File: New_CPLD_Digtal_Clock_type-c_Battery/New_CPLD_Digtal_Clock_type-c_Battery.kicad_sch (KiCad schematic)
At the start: 43 parts, among them J1 Conn_02x05_Odd_Even, J2 Conn_01x15, J3 Conn_01x15, P1 USB_C_Plug_USB2.0, Q1 CS9013, Q2 CS9013, Q3 CS9013, Q4 CS9013, SW1 SW_Push, SW2 SW_Push, SW3 SW_Push, SW4 SW_Nidec_CAS-120A1, U1 4_Digits_7Seg_CC, U2 LD1117V33, Y1 CXO_DIP8

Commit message: Add files via upload
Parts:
- added C7, C9: 0.1uF, Capacitor_SMD:C_0201_0603Metric, symbol Device:C
- added C8: 10uF, Capacitor_SMD:C_0201_0603Metric, symbol Device:C
- added D2, D3: LED, LED_SMD:LED_PLCC_2835, symbol Device:LED
- added Q5: FS8205A, SOP65P640X120-8N, symbol FS8205A:FS8205A
- added R21, R22, R25: 1k, Resistor_SMD:R_0201_0603Metric, symbol Device:R_US
- added R23: 100, Resistor_SMD:R_0201_0603Metric, symbol Device:R_US
- added R26: 1.2k, Resistor_SMD:R_0201_0603Metric, symbol Device:R_US
- added U1: EPM3064ATC100-7N, EPM3064:PLCC127P1765X1765X457-44N, symbol EPM3064:EPM3064ATC100-7N
- added U4: TP4056-42-ESOP8, Package_SO:SOIC-8-1EP_3.9x4.9mm_P1.27mm_EP2.41x3.3mm_ThermalVias, symbol TP4056:TP4056-42-ESOP8
- added U5: DW01A, Package_TO_SOT_SMD:SOT-23-6, symbol Battery_Management:DW01A
- BT1: value Battery -> 3.7V
- C1: value C -> 10uF; footprint (none) -> Capacitor_SMD:C_0201_0603Metric; Voltage (none) -> 25V
- C2, C3, C4, C5, C6: footprint (none) -> Capacitor_SMD:C_0201_0603Metric
- D1: footprint (none) -> LED_SMD:LED_PLCC_2835
- J1: footprint (none) -> Connector_IDC:IDC-Header_2x03_P2.54mm_Vertical
- J2, J3: footprint (none) -> Connector_PinHeader_1.00mm:PinHeader_1x15_P1.00mm_Vertical
- P1: footprint (none) -> Connector_USB:USB_C_Receptacle_GCT_USB4125-xx-x-0190_6P_TopMnt_Horizontal
- R1, R2, R3, R4: footprint (none) -> Resistor_SMD:R_0201_0603Metric
- R5: value R_US -> 220; footprint (none) -> Resistor_SMD:R_0201_0603Metric
- SW1, SW2, SW3: footprint (none) -> Button_Switch_THT:SW_PUSH_6mm
- SW4: footprint Button_Switch_SMD:Nidec_Copal_CAS-120A -> Button_Switch_THT:SW_Slide_SPDT_Straight_CK_OS102011MS2Q
- renumbered U1 to U3
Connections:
- net GCLK1: now also U1.43 (GCLK1)
- net GNDREF: now also BT1.2 (-), P1.A1 (GND), P1.A12 (GND), P1.B1 (GND), P1.B12 (GND), C7.2, C8.2, C9.2, Q5.2, Q5.3, Q5.6, Q5.7, R25.2, R26.2, U1.10 (GND), U1.17 (GND), U1.22 (GND), U1.30 (GND), U1.36 (GND), U1.4 (IO), U1.42 (GND), U1.5 (IO), U1.6 (IO), U4.1 (TEMP), U4.3 (GND), U5.6 (GND)
- net P11: now also U1.11 (IO)
- net P12: now also U1.12 (IO)
- net P14: now also U1.14 (IO)
- net P16: now also U1.16 (IO)
- net P18: now also U1.18 (IO)
- net P19: now also U1.19 (IO)
- net P20: now also U1.20 (IO)
- net P21: now also U1.21 (IO)
- net P24: now also U1.24 (IO)
- net P25: now also U1.25 (IO)
- net P26: now also U1.26 (IO)
- net P27: now also U1.27 (IO)
- net P28: now also U1.28 (IO)
- net P29: now also U1.29 (IO)
- net P31: now also U1.31 (IO)
- net P33: now also U1.33 (IO)
- net P34: now also U1.34 (IO)
- net P37: now also U1.37 (IO)
- net P39: now also U1.39 (IO)
- net P40: now also U1.40 (IO)
- net P41: now also U1.41 (IO)
- net P8: now also U1.8 (IO)
- net P9: now also U1.9 (IO)
- net TCK: now also U1.32 (TCK)
- net TDI: now also U1.7 (TDI)
- net TDO: now also U1.38 (TDO)
- net TMS: now also U1.13 (TMS)
- net VCC: now also SW4.3 (A), U1.15 (VCC), U1.23 (VCC), U1.3 (VCC), U1.35 (VCC); no longer U2.2 (VO)
- net at BT1.1 (+), U2.3 (VI): now also C8.1, R23.1, U4.5 (BAT)
- net at P1.A5 (CC): now also C7.1, D2.2 (A), D3.2 (A)
- new net: D2.1 (K), R21.1
- new net: R21.2, U4.7 (~{CHRG})
- new net: R26.1, U4.2 (PROG)
- new net: R22.2, U4.6 (~{STDBY})
- new net: C9.1, R23.2, U5.5 (VCC)
- new net: R25.1, U5.2 (CS)
- new net: Q5.1, Q5.8
- new net: Q5.4, U5.1 (OD)
- new net: Q5.5, U5.3 (OC)
- new net: D3.1 (K), R22.1
- new net GCLK2: U1.2 (GCLK2)
- new net GCLKRn: U1.1 (GCLRn)
- new net OE1: U1.44 (OE1)
- new net OUT+: U2.2 (VO)
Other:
- moved on the sheet: BT1, C1, D1, J3, P1, Q1, Q2, Q3, Q4, R10, R11, R12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

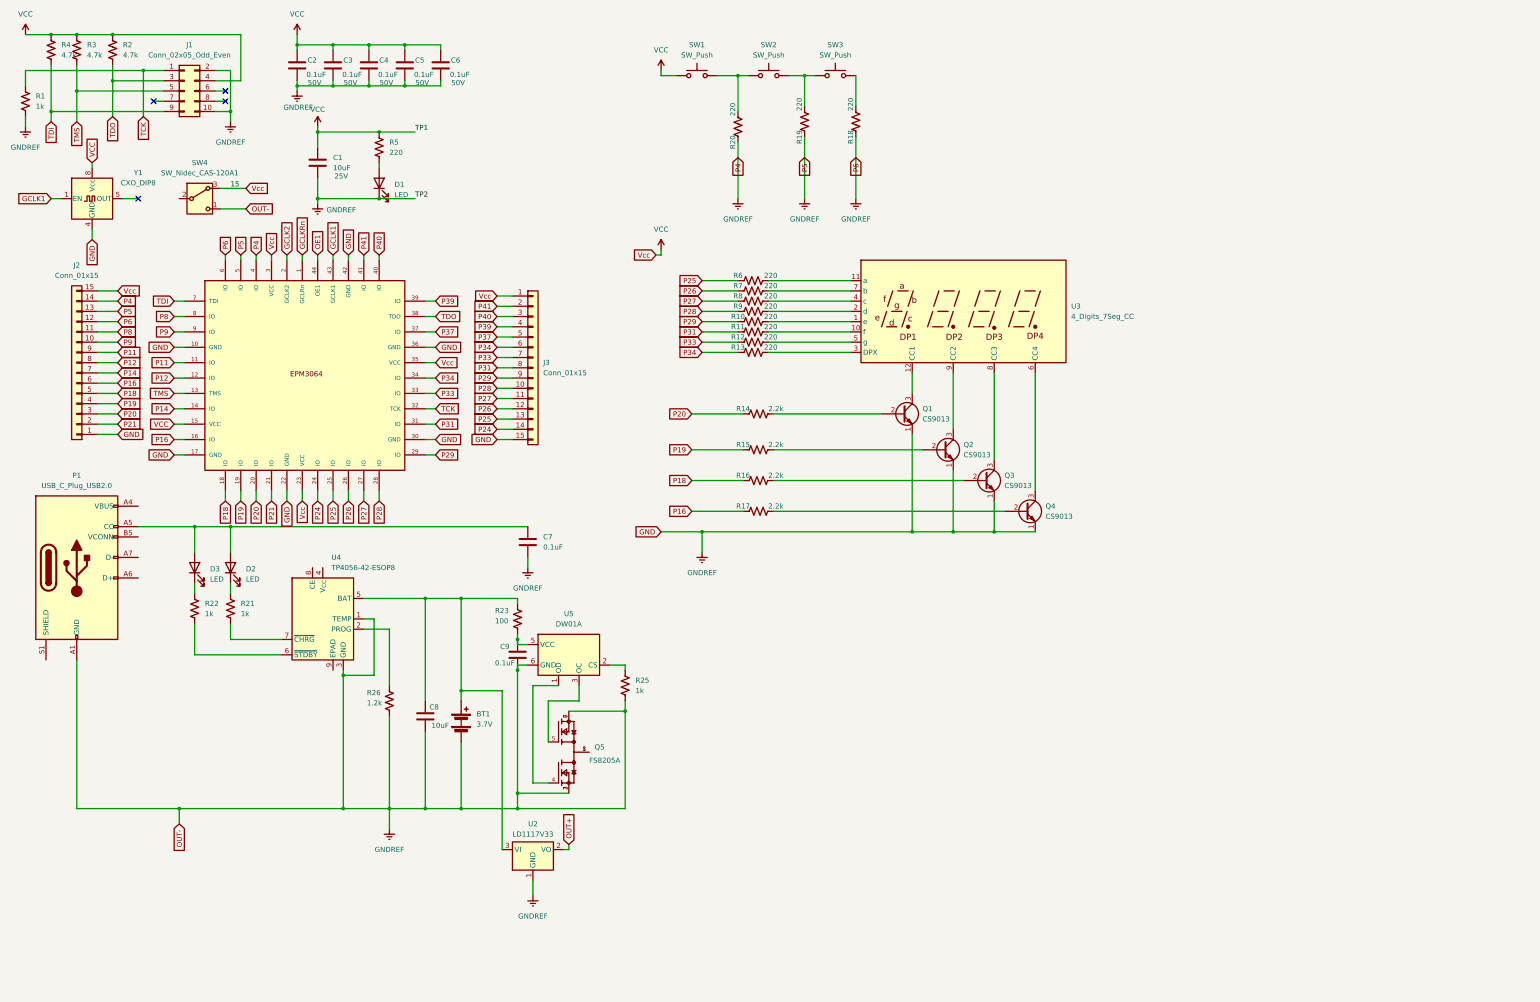
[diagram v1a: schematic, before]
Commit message: Add files via upload
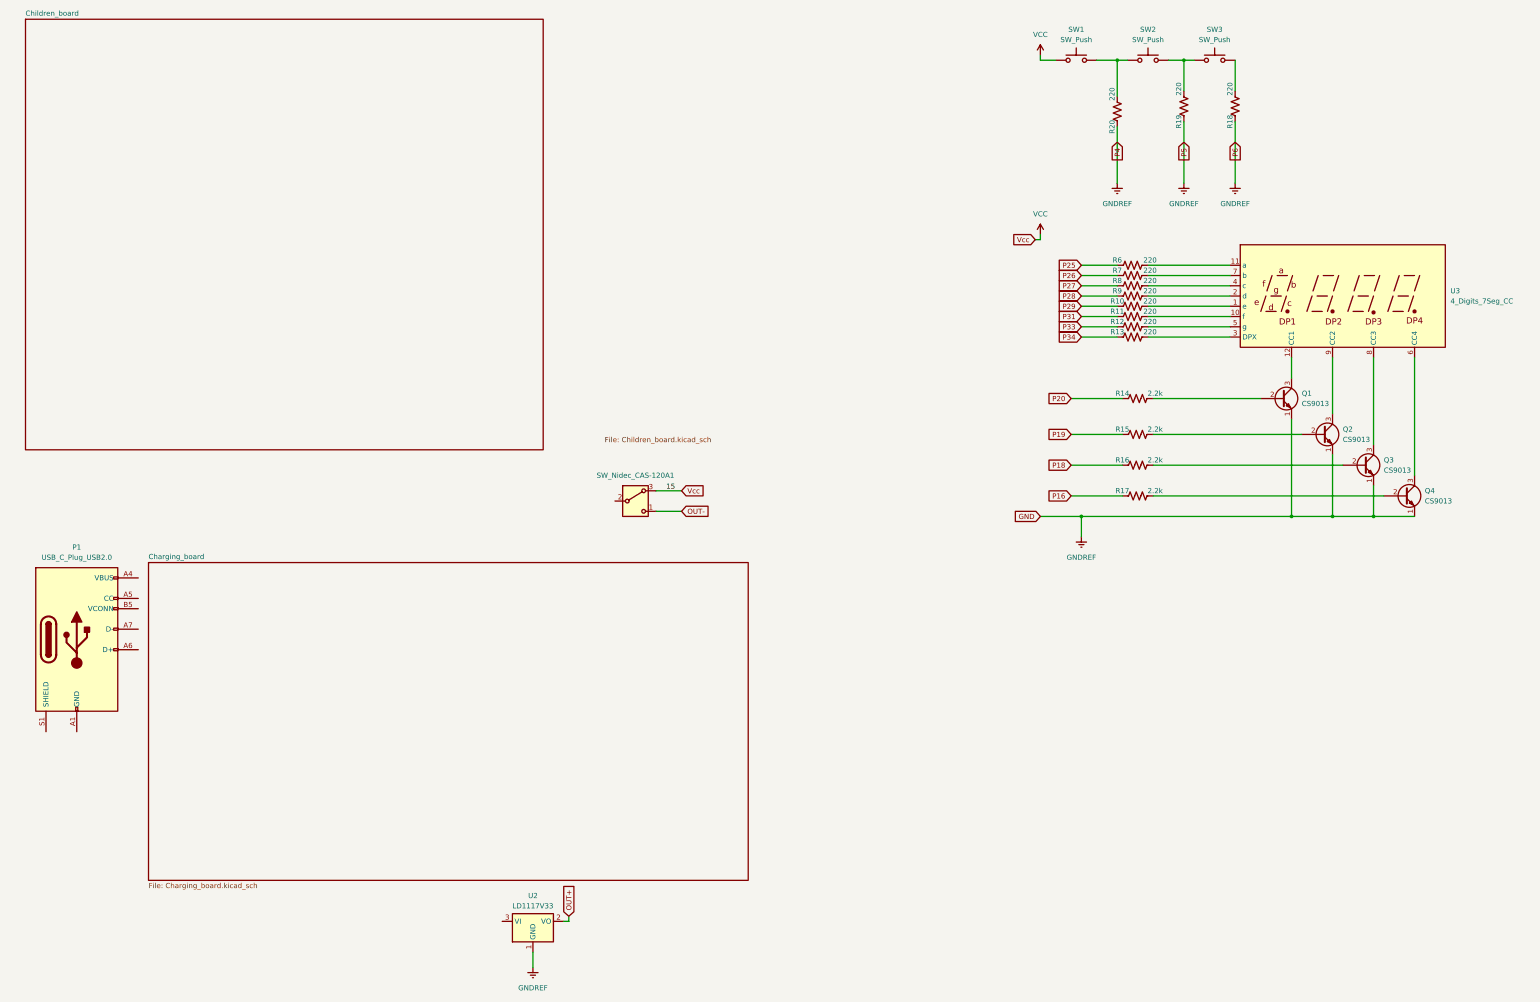
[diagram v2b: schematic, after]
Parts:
- removed BT1: 3.7V, symbol Device:Battery
- removed C1, C8: 10uF, Capacitor_SMD:C_0201_0603Metric, symbol Device:C
- removed C2, C3, C4, C5, C6, C7, C9: 0.1uF, Capacitor_SMD:C_0201_0603Metric, symbol Device:C
- removed D1, D2, D3: LED, LED_SMD:LED_PLCC_2835, symbol Device:LED
- removed J1: Conn_02x05_Odd_Even, Connector_IDC:IDC-Header_2x03_P2.54mm_Vertical, symbol Connector_Generic:Conn_02x05_Odd_Even
- removed J2, J3: Conn_01x15, Connector_PinHeader_1.00mm:PinHeader_1x15_P1.00mm_Vertical, symbol Connector_Generic:Conn_01x15
- removed Q5: FS8205A, SOP65P640X120-8N, symbol FS8205A:FS8205A
- removed R1, R21, R22, R25: 1k, Resistor_SMD:R_0201_0603Metric, symbol Device:R_US
- removed R2, R3, R4: 4.7k, Resistor_SMD:R_0201_0603Metric, symbol Device:R_US
- removed R23: 100, Resistor_SMD:R_0201_0603Metric, symbol Device:R_US
- removed R26: 1.2k, Resistor_SMD:R_0201_0603Metric, symbol Device:R_US
- removed R5: 220, Resistor_SMD:R_0201_0603Metric, symbol Device:R_US
- removed U1: EPM3064ATC100-7N, EPM3064:PLCC127P1765X1765X457-44N, symbol EPM3064:EPM3064ATC100-7N
- removed U4: TP4056-42-ESOP8, Package_SO:SOIC-8-1EP_3.9x4.9mm_P1.27mm_EP2.41x3.3mm_ThermalVias, symbol TP4056:TP4056-42-ESOP8
- removed U5: DW01A, Package_TO_SOT_SMD:SOT-23-6, symbol Battery_Management:DW01A
- removed Y1: CXO_DIP8, Oscillator:Oscillator_DIP-8, symbol Oscillator:CXO_DIP8
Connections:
- net GNDREF: no longer P1.A1 (GND), P1.A12 (GND), P1.B1 (GND), P1.B12 (GND), SW4.1 (C)
- new net: P1.A1 (GND), P1.A12 (GND), P1.B1 (GND), P1.B12 (GND)
- new net OUT-: SW4.1 (C)
- no-connect marks 4 -> 0
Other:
- added sheet Charging_board (Charging_board.kicad_sch)
- added sheet Children_board (Children_board.kicad_sch)
- moved on the sheet: P1, Q1, Q2, Q3, Q4, R10, R11, R12, R13, R14, R15, R16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
